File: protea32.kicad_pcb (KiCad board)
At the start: 2 copper layers, 68 x 66.5 mm, 146 parts, among them IC1 ESP32-D0WD-V3, J1 USB4215-03-A, J11 DC3RX19JA2, J2 676430910, J3 TTL, J4 D-SUB 9 Male, J5 0475710001, J6 Flash, Q1 2N7000, Q2 2N7000, Q3 2N7000, Q4 2N7000, Q5 2N7000, Q6 UMH3N, U10 W25Q32JVSIQ, U11 74HC4052D, U12 74HC4052D, U14 CH340C, U3 USBLC6-2SC6, U4 TS3USB221RSER, U5 NCP1117 3.3, U6 USBLC6-2SC6, U7 RP2040, U8 W25Q16JVSSIQ, U9 MAX232CSE+, Y2 ASE-12MHz, Y3 40MHz

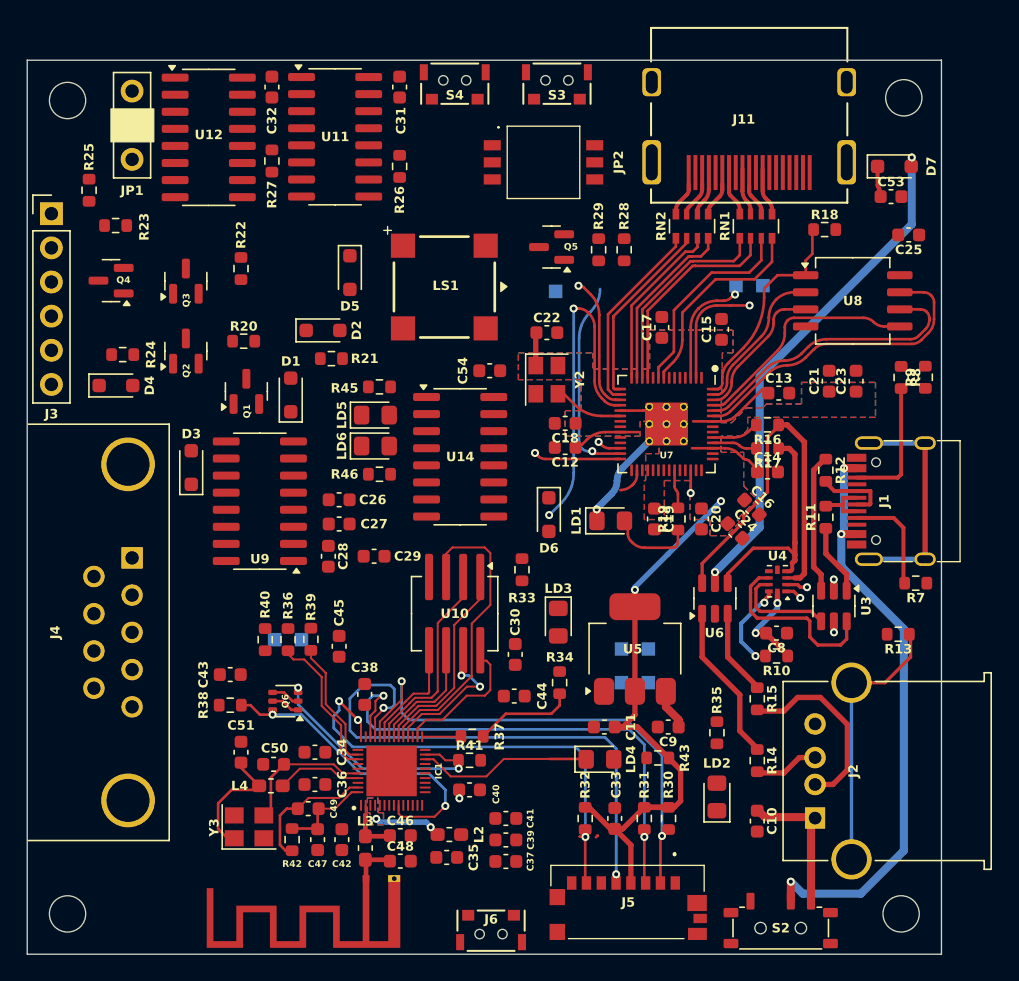
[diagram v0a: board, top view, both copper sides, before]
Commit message: Routing WIP
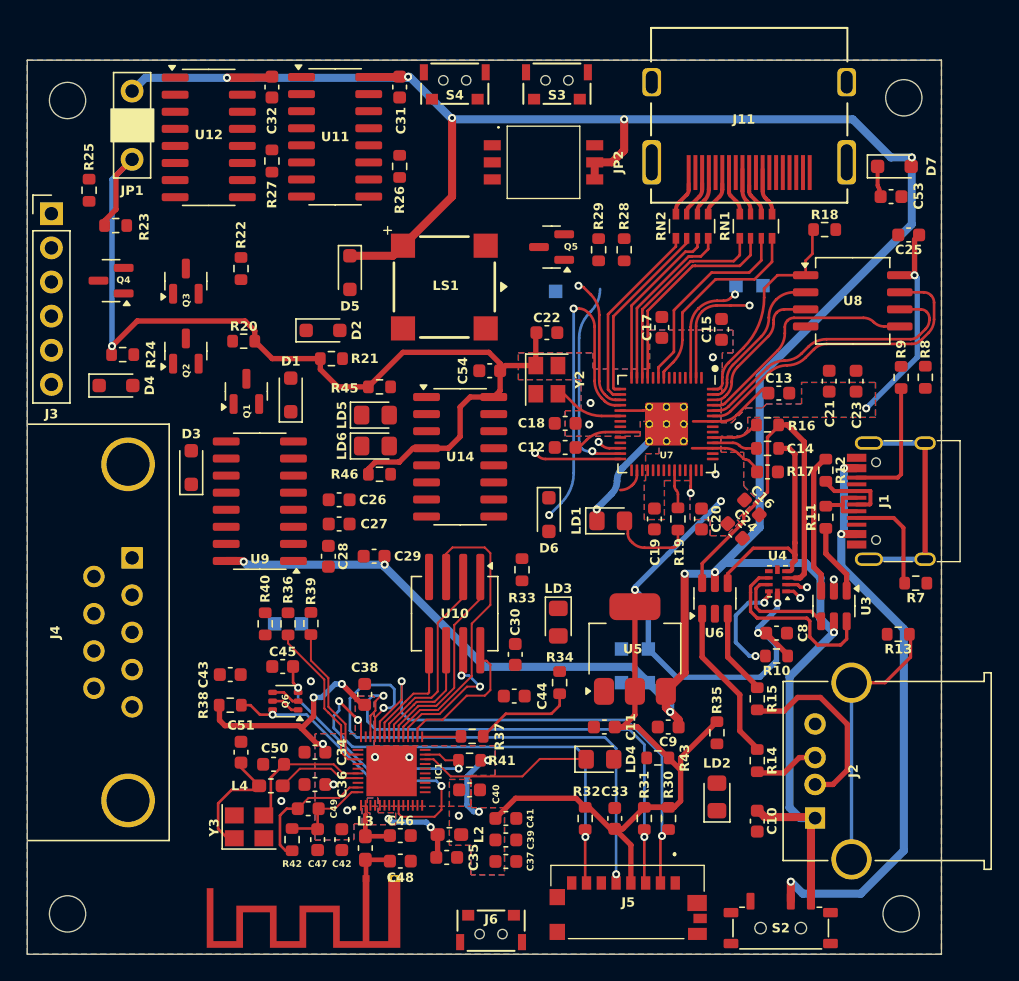
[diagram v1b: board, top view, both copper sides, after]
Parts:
- moved C45 4.46 mm to (183.7, 107.6), turned to 180 degrees
- moved J7 1.17 mm to (185.1, 104.4)
- moved R36 1.17 mm to (184.1, 104.4)
- moved R39 1.17 mm to (185.8, 104.4)
- moved R40 1.17 mm to (182.4, 104.4)
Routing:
- net VBUS: track 51.1 -> 218.5 mm, vias 3 -> 11
- net +3V3: track 50.6 -> 192.3 mm, vias 5 -> 20
- net /ESP_GPIO0: track 18.4 -> 20.0 mm
- net /UMP_SW: track 6.24 -> 7.43 mm
- net /ESP_U0RXD: track 9.57 -> 10.7 mm
- net +3.3VP: track 4.33 -> 5.17 mm
- net Net-(IC1-U0TXD): track 11.1 -> 11.8 mm
- net GND: vias 2 -> 6
- added copper zone on B.Cu, net GND
- added copper zone on F.Cu, net GND
